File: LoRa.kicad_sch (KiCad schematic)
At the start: 26 parts, among them J2 SMA_Conn, Q1 BSS84, Q2 BSS84, SW1 RST, U4 CORE1262-868M

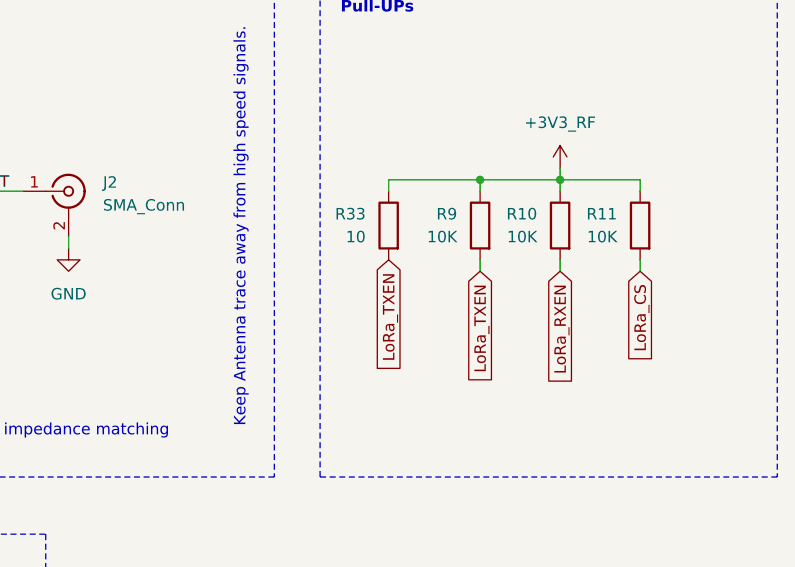
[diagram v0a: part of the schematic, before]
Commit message: reverted back to og files
[local revision r5 4274e03a1d0e]
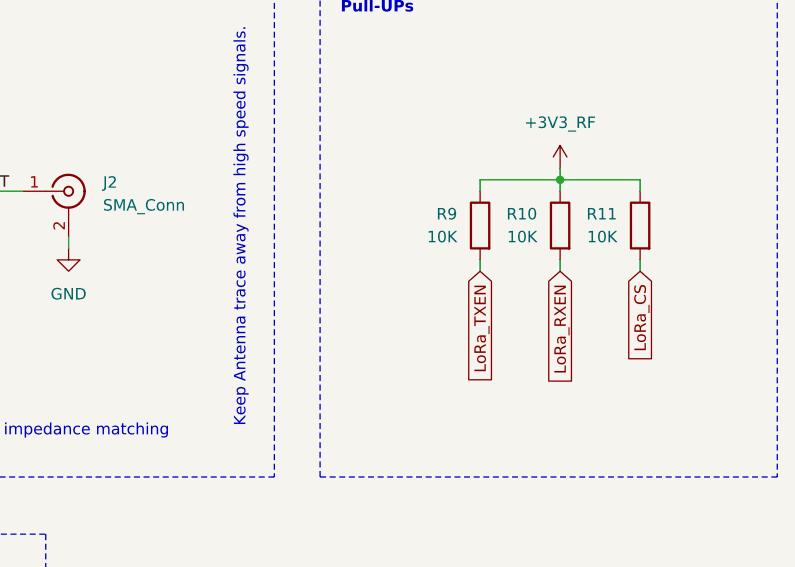
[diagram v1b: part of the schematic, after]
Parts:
- removed R33: 10, symbol Device:R
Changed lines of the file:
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@@
 		(color 0 0 0 0)
 	)
-	(junction
-		(at 245.11 40.64)
-		(diameter 0)
-		(color 0 0 0 0)
-	)
 	(wire
 		(pts
@@
 	(wire
 		(pts
-			(xy 234.95 41.91) (xy 234.95 40.64)
-		)
-		(stroke
-			(width 0)
-			(type default)
-		)
-	)
-	(wire
-		(pts
 			(xy 254 39.37) (xy 254 40.64)
 		)
@@
 	(wire
 		(pts
-			(xy 234.95 40.64) (xy 245.11 40.64)
-		)
-		(stroke
-			(width 0)
-			(type default)
-		)
-	)
-	(wire
-		(pts
 			(xy 87.63 104.14) (xy 90.17 104.14)
 		)
@@
 		)
 	)
-	(global_label "LoRa_TXEN"
-		(shape input)
-		(at 234.95 49.53 270)
-		(fields_autoplaced yes)
-		(effects
-			(font
-				(size 1.27 1.27)
-				(thickness 0.1588)
-			)
-			(justify right)
-		)
-		(property "Intersheetrefs" "${INTERSHEET_REFS}"
-			(at 234.95 62.7355 90)
-			(hide yes)
-			(show_name no)
-			(do_not_autoplace no)
-			(effects
-				(font
-					(size 1.27 1.27)
-				)
-				(justify right)
-			)
-		)
-	)
 	(global_label "DIO2"
 		(shape input)
@@
 					(unit 1)
 				)
-			)
-		)
-	)
-	(symbol
-		(lib_id "Device:R")
-		(at 234.95 45.72 0)
-		(mirror y)
-		(unit 1)
-		(body_style 1)
-		(exclude_from_sim no)
-		(in_bom yes)
-		(on_board yes)
-		(in_pos_files yes)
-		(dnp no)
-		(property "Reference" "R33"
-			(at 232.41 44.4499 0)
-			(show_name no)
-			(do_not_autoplace no)
-			(effects
-				(font
-					(size 1.27 1.27)
-				)
-				(justify left)
-			)
-		)
-		(property "Value" "10"
-			(at 232.41 46.9899 0)
-			(show_name no)
-			(do_not_autoplace no)
-			(effects
-				(font
-					(size 1.27 1.27)
-				)
-				(justify left)
-			)
-		)
-		(property "Footprint" ""
-			(at 236.728 45.72 90)
-			(hide yes)
-			(show_name no)
-			(do_not_autoplace no)
-			(effects
-				(font
-					(size 1.27 1.27)
-				)
-			)
-		)
-		(property "Datasheet" ""
-			(at 234.95 45.72 0)
-			(hide yes)
-			(show_name no)
-			(do_not_autoplace no)
-			(effects
-				(font
-					(size 1.27 1.27)
-				)
-			)
-		)
-		(property "Description" "Resistor"
-			(at 234.95 45.72 0)
-			(hide yes)
-			(show_name no)
-			(do_not_autoplace no)
-			(effects
-				(font
-					(size 1.27 1.27)
-				)
-			)
-		)
-		(pin "1"
-		)
-		(pin "2"
-		)
-		(instances
-			(project "Demo Project"
-				(path "/4e55511c-c365-4512-9b57-837a9ec6e386/e05efdcd-bdb1-4ad7-9946-40f9f2f2fdae"
-					(reference "R33")
-					(unit 1)
-				)

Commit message: testing plugin
[local revision r3 cb60daacd4a3]
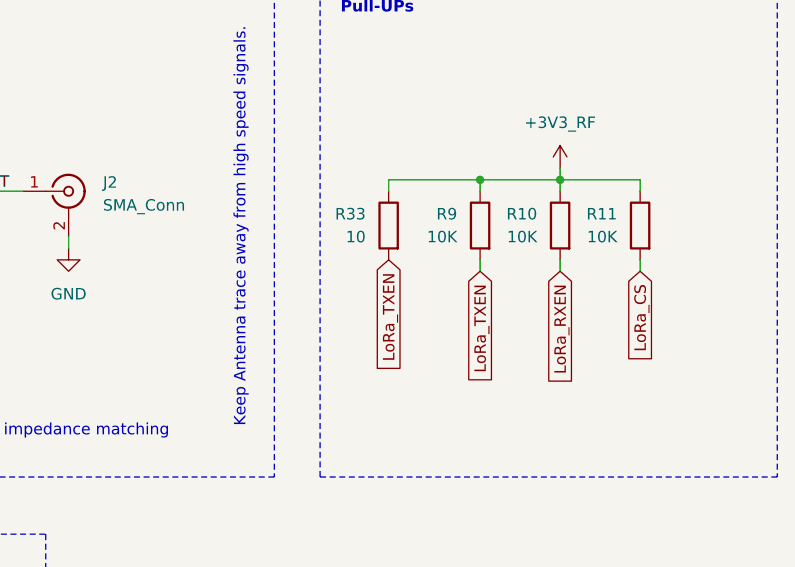
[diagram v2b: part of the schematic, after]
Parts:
- added R33: 10, symbol Device:R
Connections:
- net +3V3: now also R33.1
- net LoRa_TXEN: now also R33.2
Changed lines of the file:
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@@
 		(color 0 0 0 0)
 	)
+	(junction
+		(at 245.11 40.64)
+		(diameter 0)
+		(color 0 0 0 0)
+	)
 	(wire
 		(pts
@@
 	(wire
 		(pts
+			(xy 234.95 41.91) (xy 234.95 40.64)
+		)
+		(stroke
+			(width 0)
+			(type default)
+		)
+	)
+	(wire
+		(pts
 			(xy 254 39.37) (xy 254 40.64)
 		)
@@
 	(wire
 		(pts
+			(xy 234.95 40.64) (xy 245.11 40.64)
+		)
+		(stroke
+			(width 0)
+			(type default)
+		)
+	)
+	(wire
+		(pts
 			(xy 87.63 104.14) (xy 90.17 104.14)
 		)
@@
 		)
 	)
+	(global_label "LoRa_TXEN"
+		(shape input)
+		(at 234.95 49.53 270)
+		(fields_autoplaced yes)
+		(effects
+			(font
+				(size 1.27 1.27)
+				(thickness 0.1588)
+			)
+			(justify right)
+		)
+		(property "Intersheetrefs" "${INTERSHEET_REFS}"
+			(at 234.95 62.7355 90)
+			(hide yes)
+			(show_name no)
+			(do_not_autoplace no)
+			(effects
+				(font
+					(size 1.27 1.27)
+				)
+				(justify right)
+			)
+		)
+	)
 	(global_label "DIO2"
 		(shape input)
@@
 					(unit 1)
 				)
+			)
+		)
+	)
+	(symbol
+		(lib_id "Device:R")
+		(at 234.95 45.72 0)
+		(mirror y)
+		(unit 1)
+		(body_style 1)
+		(exclude_from_sim no)
+		(in_bom yes)
+		(on_board yes)
+		(in_pos_files yes)
+		(dnp no)
+		(property "Reference" "R33"
+			(at 232.41 44.4499 0)
+			(show_name no)
+			(do_not_autoplace no)
+			(effects
+				(font
+					(size 1.27 1.27)
+				)
+				(justify left)
+			)
+		)
+		(property "Value" "10"
+			(at 232.41 46.9899 0)
+			(show_name no)
+			(do_not_autoplace no)
+			(effects
+				(font
+					(size 1.27 1.27)
+				)
+				(justify left)
+			)
+		)
+		(property "Footprint" ""
+			(at 236.728 45.72 90)
+			(hide yes)
+			(show_name no)
+			(do_not_autoplace no)
+			(effects
+				(font
+					(size 1.27 1.27)
+				)
+			)
+		)
+		(property "Datasheet" ""
+			(at 234.95 45.72 0)
+			(hide yes)
+			(show_name no)
+			(do_not_autoplace no)
+			(effects
+				(font
+					(size 1.27 1.27)
+				)
+			)
+		)
+		(property "Description" "Resistor"
+			(at 234.95 45.72 0)
+			(hide yes)
+			(show_name no)
+			(do_not_autoplace no)
+			(effects
+				(font
+					(size 1.27 1.27)
+				)
+			)
+		)
+		(pin "1"
+		)
+		(pin "2"
+		)
+		(instances
+			(project "Demo Project"
+				(path "/4e55511c-c365-4512-9b57-837a9ec6e386/e05efdcd-bdb1-4ad7-9946-40f9f2f2fdae"
+					(reference "R33")
+					(unit 1)
+				)
